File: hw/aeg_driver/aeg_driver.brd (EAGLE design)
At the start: 37 x 48 mm, 48 parts, among them J1 JST-ZH6SMT_VERT, J2 XT30XT30PW_MALE, U1 MAX150628TDFN, U2 TCAN334GSOT23, U3 STM32G474CEU6, U4 MC33926, U5 MC33926

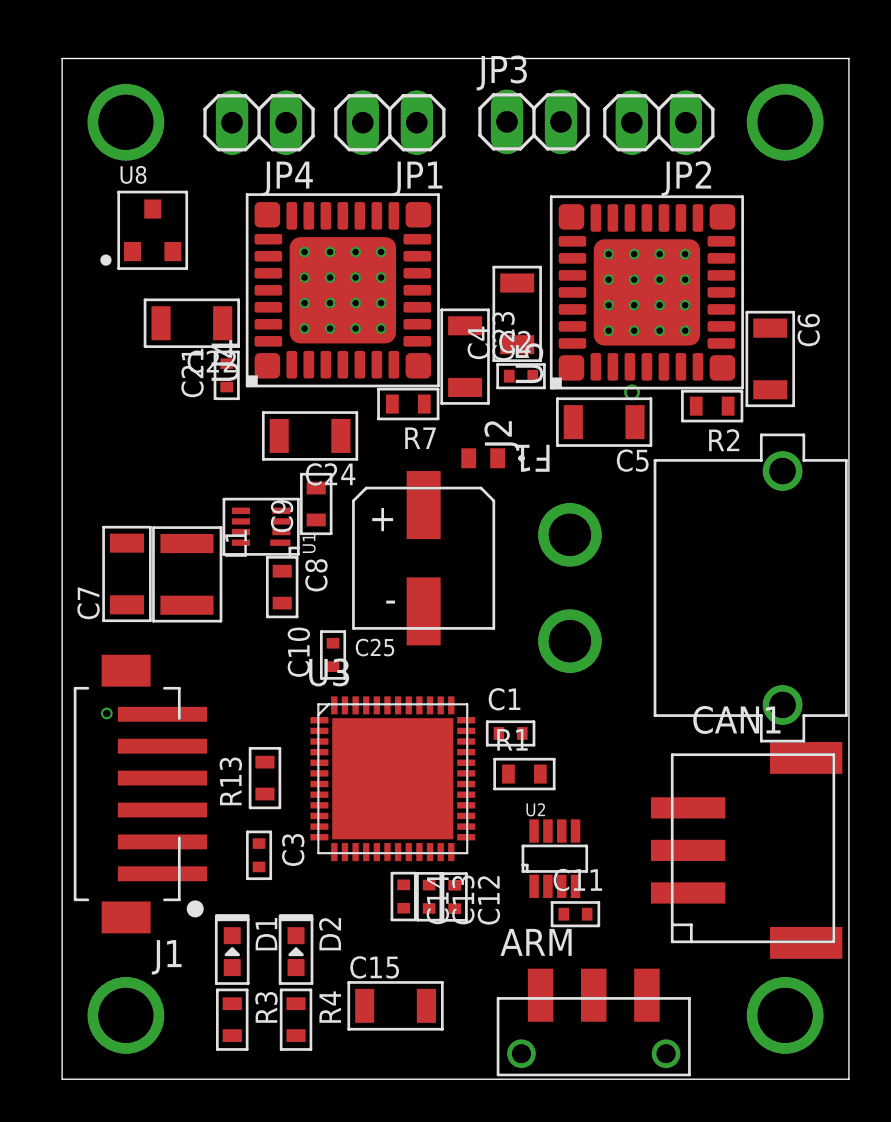
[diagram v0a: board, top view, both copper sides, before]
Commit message: Checkpoint of aeg_driver
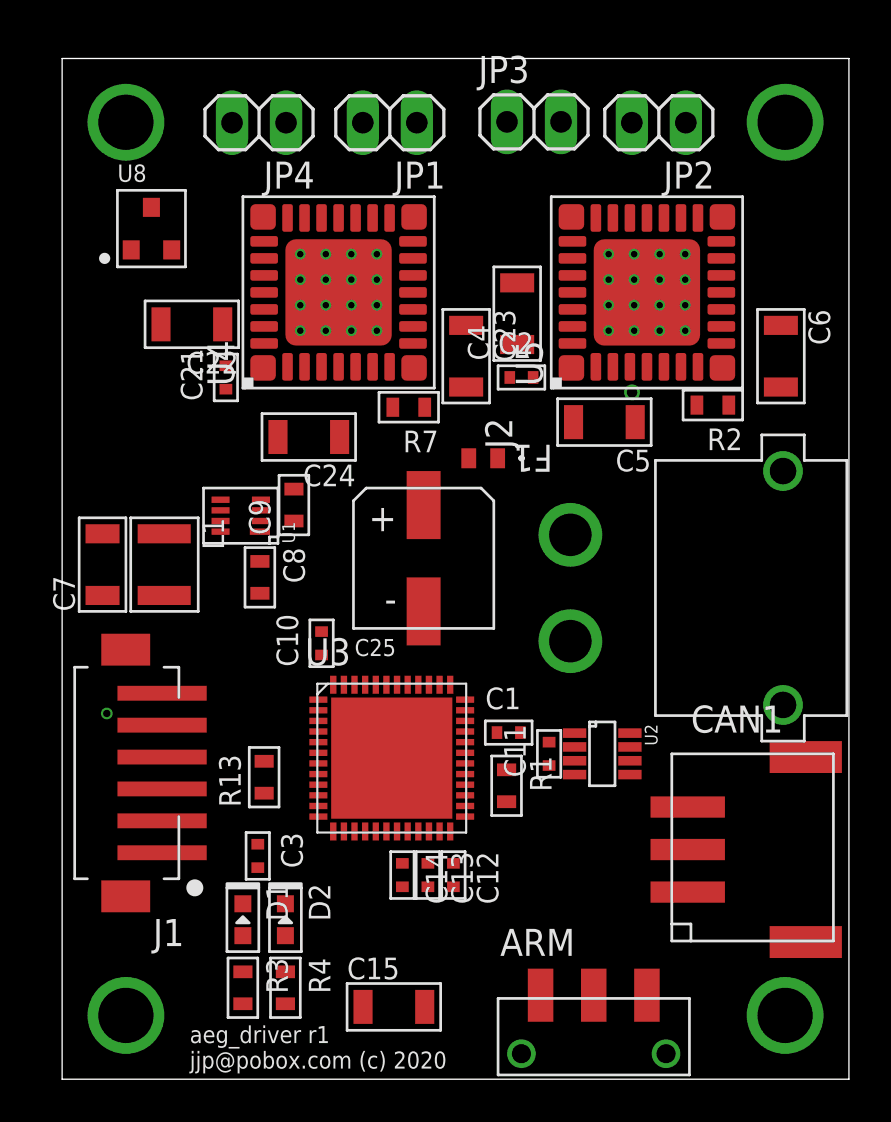
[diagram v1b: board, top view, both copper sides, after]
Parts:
- moved C11 7.64 mm to (22.9, 15.3), turned to 90 degrees
- moved U2 5.41 mm to (25.4, 15.3), turned to 270 degrees
- moved D1 1.58 mm to (8.50, 7.50)
- moved D2 1.58 mm to (10.5, 7.50)
- moved R3 1.58 mm to (8.50, 4.30)
- moved R4 1.58 mm to (10.5, 4.30)
- moved C7 1.23 mm to (1.90, 24.2)
- moved L1 1.16 mm to (4.80, 24.2)
- moved C8 1.15 mm to (9.30, 23.6)
- moved U1 1.09 mm to (8.40, 26.5)
- moved C9 1.05 mm to (10.9, 27.0)
- moved C12 1.03 mm to (18.4, 9.60)
- moved C13 1.02 mm to (17.2, 9.60)
- moved C14 1.01 mm to (16.0, 9.60)
- moved R1 1.00 mm to (20.9, 13.8), turned to 270 degrees
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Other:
- board text added: "aeg_driver r1 jjp@pobox.com (c) 2020"
